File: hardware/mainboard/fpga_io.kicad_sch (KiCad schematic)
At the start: 24 parts, among them U1 LIFCL_40_CABGA400, X1 XO32

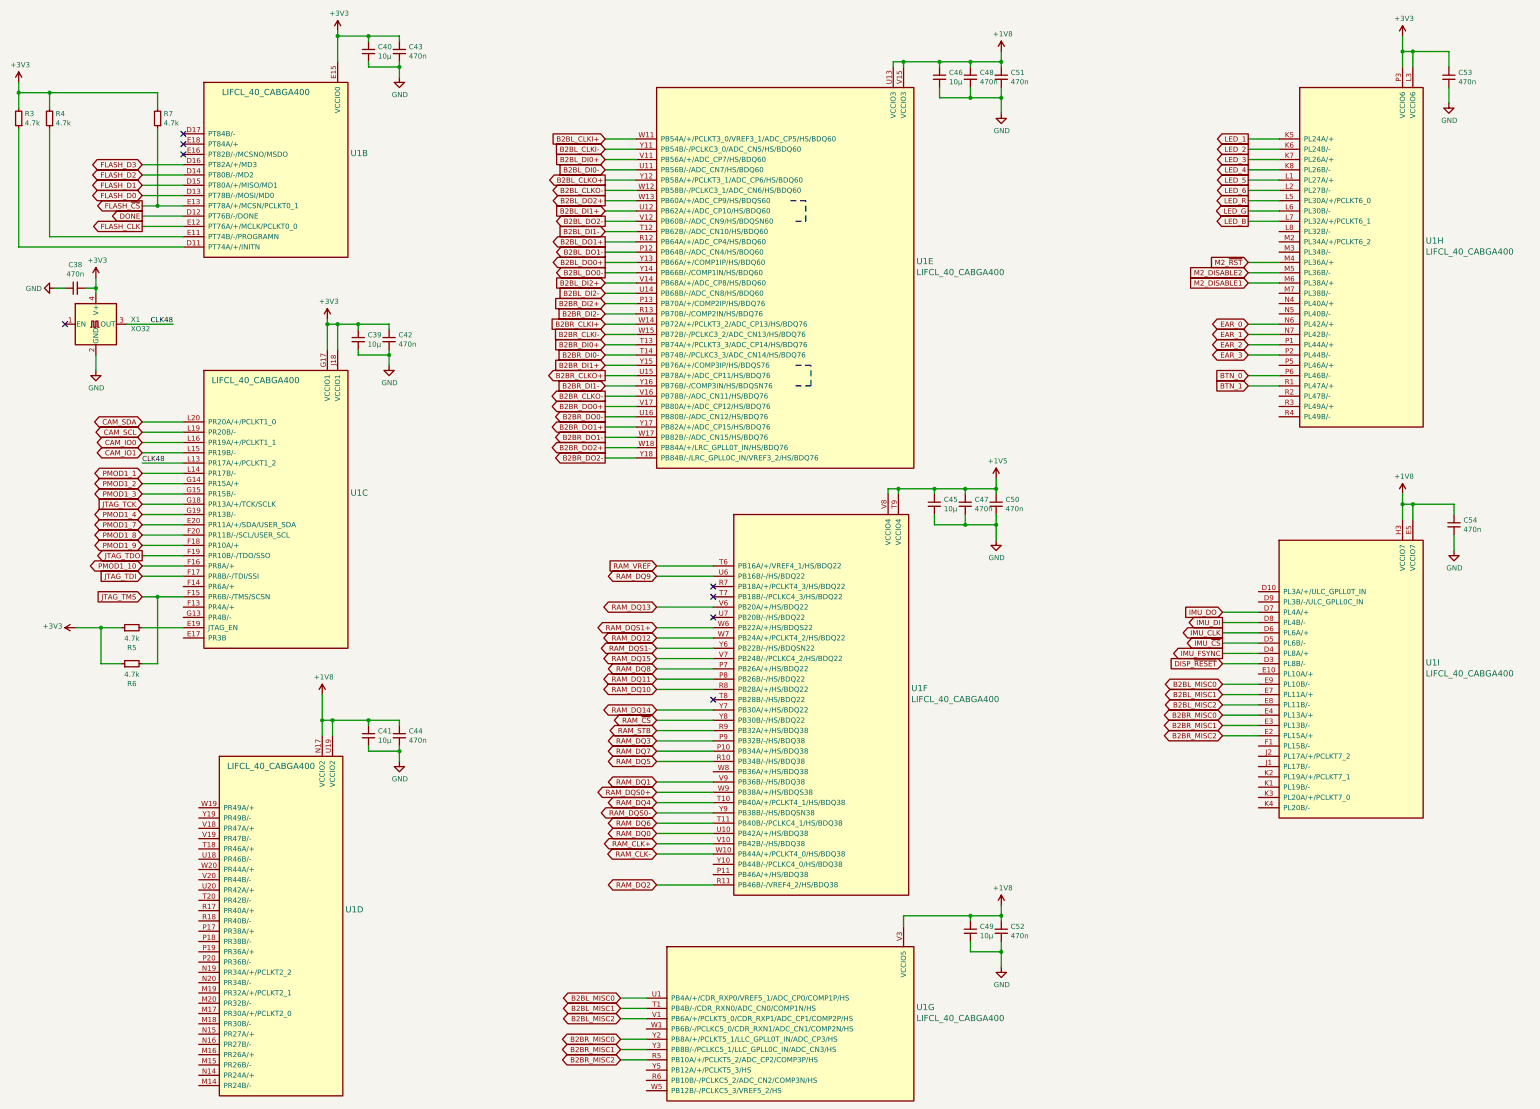
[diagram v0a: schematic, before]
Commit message: More misc routing
Signed-off-by: David Shah <dave@ds0.me>
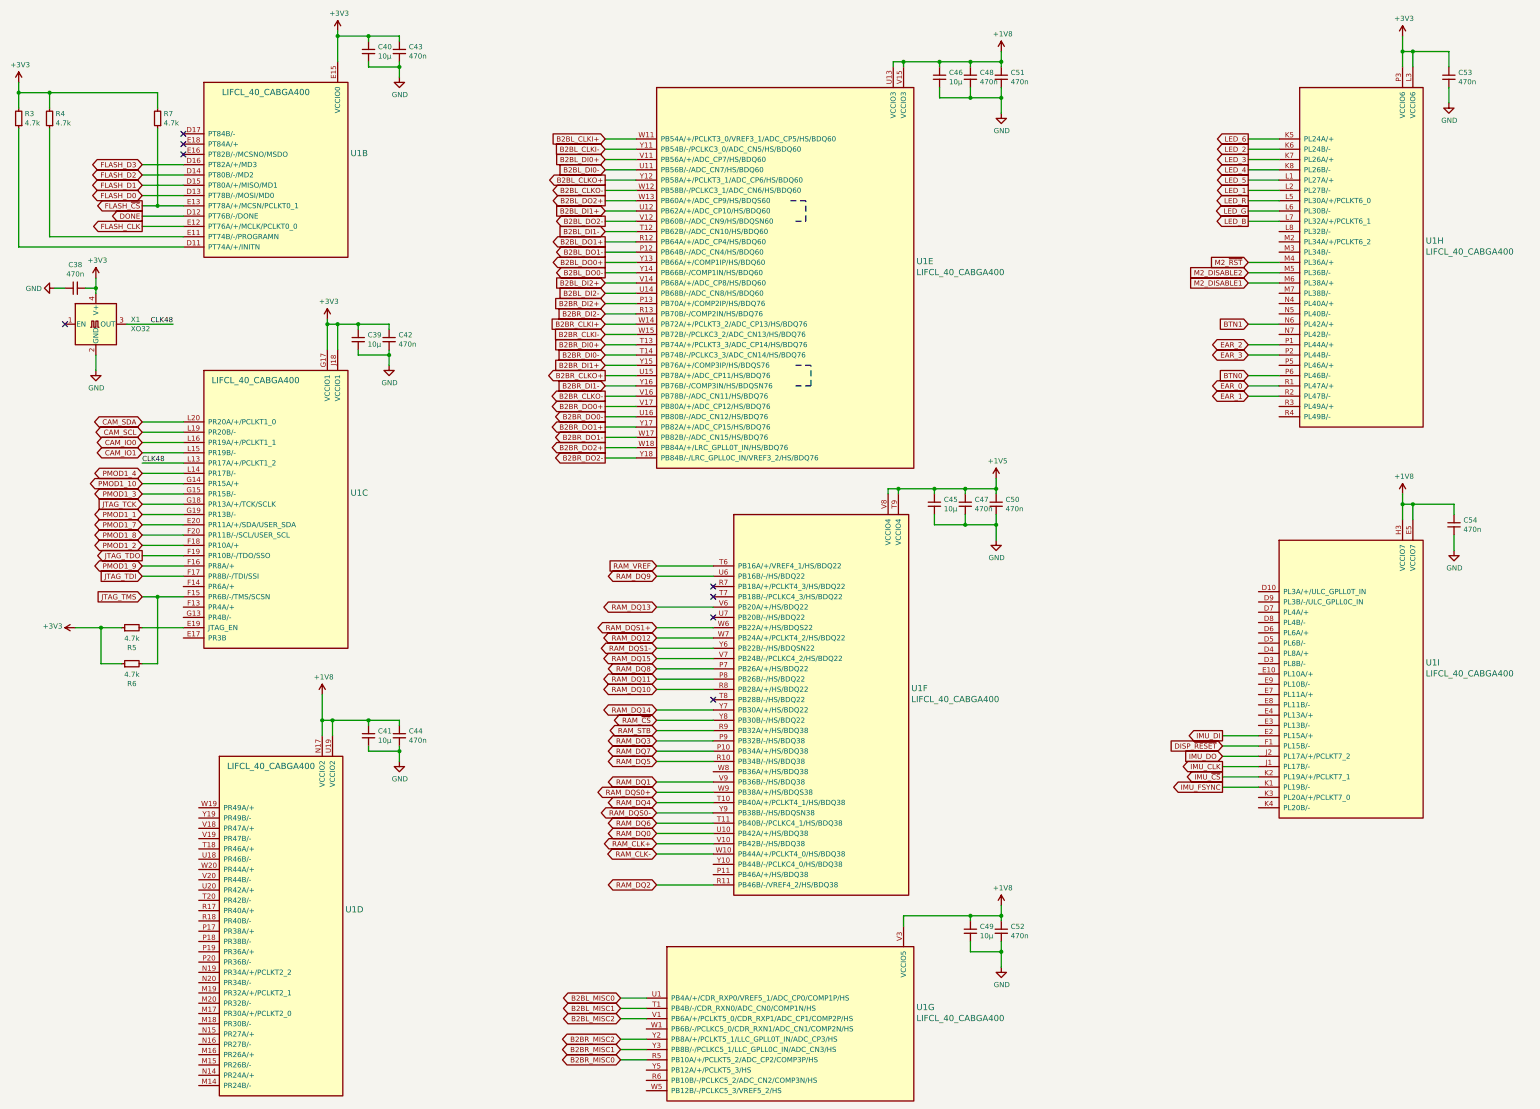
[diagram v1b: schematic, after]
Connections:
- net BTN_1 is gone; now on net EAR_0: U1.R1 (PL47A/+)
- net B2BL_MISC0: no longer U1.E9 (PL10B/-)
- net B2BL_MISC1: no longer U1.E7 (PL11A/+)
- net B2BL_MISC2: no longer U1.E8 (PL11B/-)
- net B2BR_MISC0: now also U1.R5 (PB10A/+/PCLKT5_2/ADC_CP2/COMP3P/HS); no longer U1.E4 (PL13A/+), U1.Y2 (PB8A/+/PCLKT5_1/LLC_GPLL0T_IN/ADC_CP3/HS)
- net B2BR_MISC1: no longer U1.E3 (PL13B/-)
- net B2BR_MISC2: now also U1.Y2 (PB8A/+/PCLKT5_1/LLC_GPLL0T_IN/ADC_CP3/HS); no longer U1.E2 (PL15A/+), U1.R5 (PB10A/+/PCLKT5_2/ADC_CP2/COMP3P/HS)
- net DISP_~RESET: now also U1.F1 (PL15B/-); no longer U1.D3 (PL8B/-)
- net EAR_0: no longer U1.N6 (PL42A/+)
- net EAR_1: now also U1.R2 (PL47B/-); no longer U1.N7 (PL42B/-)
- net IMU_CLK: now also U1.J1 (PL17B/-); no longer U1.D6 (PL6A/+)
- net IMU_DI: now also U1.E2 (PL15A/+); no longer U1.D8 (PL4B/-)
- net IMU_DO: now also U1.J2 (PL17A/+/PCLKT7_2); no longer U1.D7 (PL4A/+)
- net IMU_FSYNC: now also U1.K1 (PL19B/-); no longer U1.D4 (PL8A/+)
- net IMU_~CS: now also U1.K2 (PL19A/+/PCLKT7_1); no longer U1.D5 (PL6B/-)
- net LED_1: now also U1.L2 (PL27B/-); no longer U1.K5 (PL24A/+)
- net LED_6: now also U1.K5 (PL24A/+); no longer U1.L2 (PL27B/-)
- net PMOD1_1: now also U1.G19 (PR13B/-); no longer U1.L14 (PR17B/-)
- net PMOD1_10: now also U1.G14 (PR15A/+); no longer U1.F16 (PR8A/+)
- net PMOD1_2: now also U1.F18 (PR10A/+); no longer U1.G14 (PR15A/+)
- net PMOD1_4: now also U1.L14 (PR17B/-); no longer U1.G19 (PR13B/-)
- net PMOD1_9: now also U1.F16 (PR8A/+); no longer U1.F18 (PR10A/+)
- net BTN_0 renamed BTN0
- new net BTN1: U1.N6 (PL42A/+)
